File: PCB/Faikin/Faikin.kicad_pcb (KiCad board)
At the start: 2 copper layers, 70 x 70 mm, 44 parts, among them J1 1x5, J2 TC2030-USB-NL, J3 Reset, Q1 BSS138PS, U1 TPS562246, U4 ESP32-S3-MINI-1

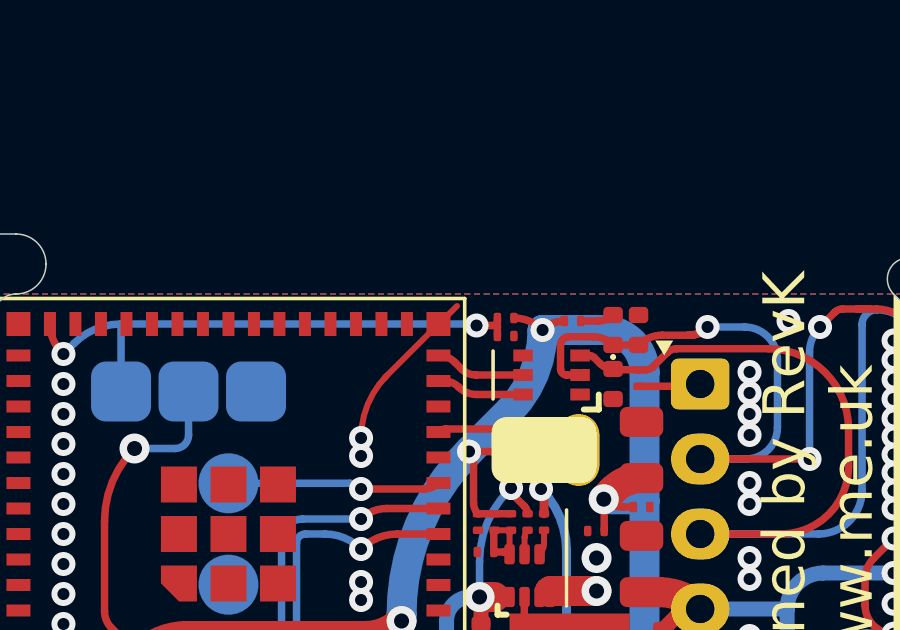
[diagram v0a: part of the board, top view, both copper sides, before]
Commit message: Track adjust
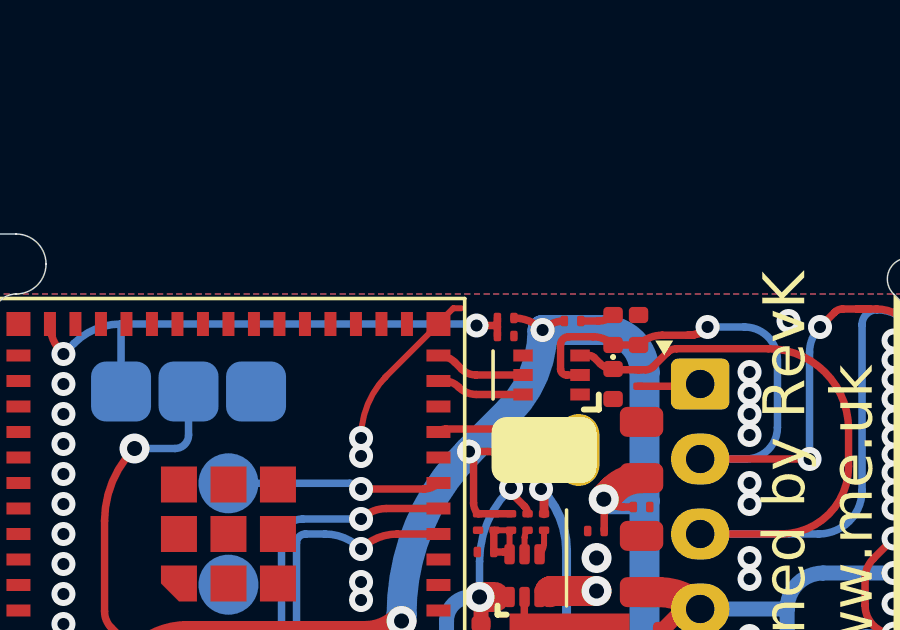
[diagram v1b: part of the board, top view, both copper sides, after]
